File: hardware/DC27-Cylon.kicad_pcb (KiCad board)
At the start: 2 copper layers, 79 x 102 mm, 3 parts

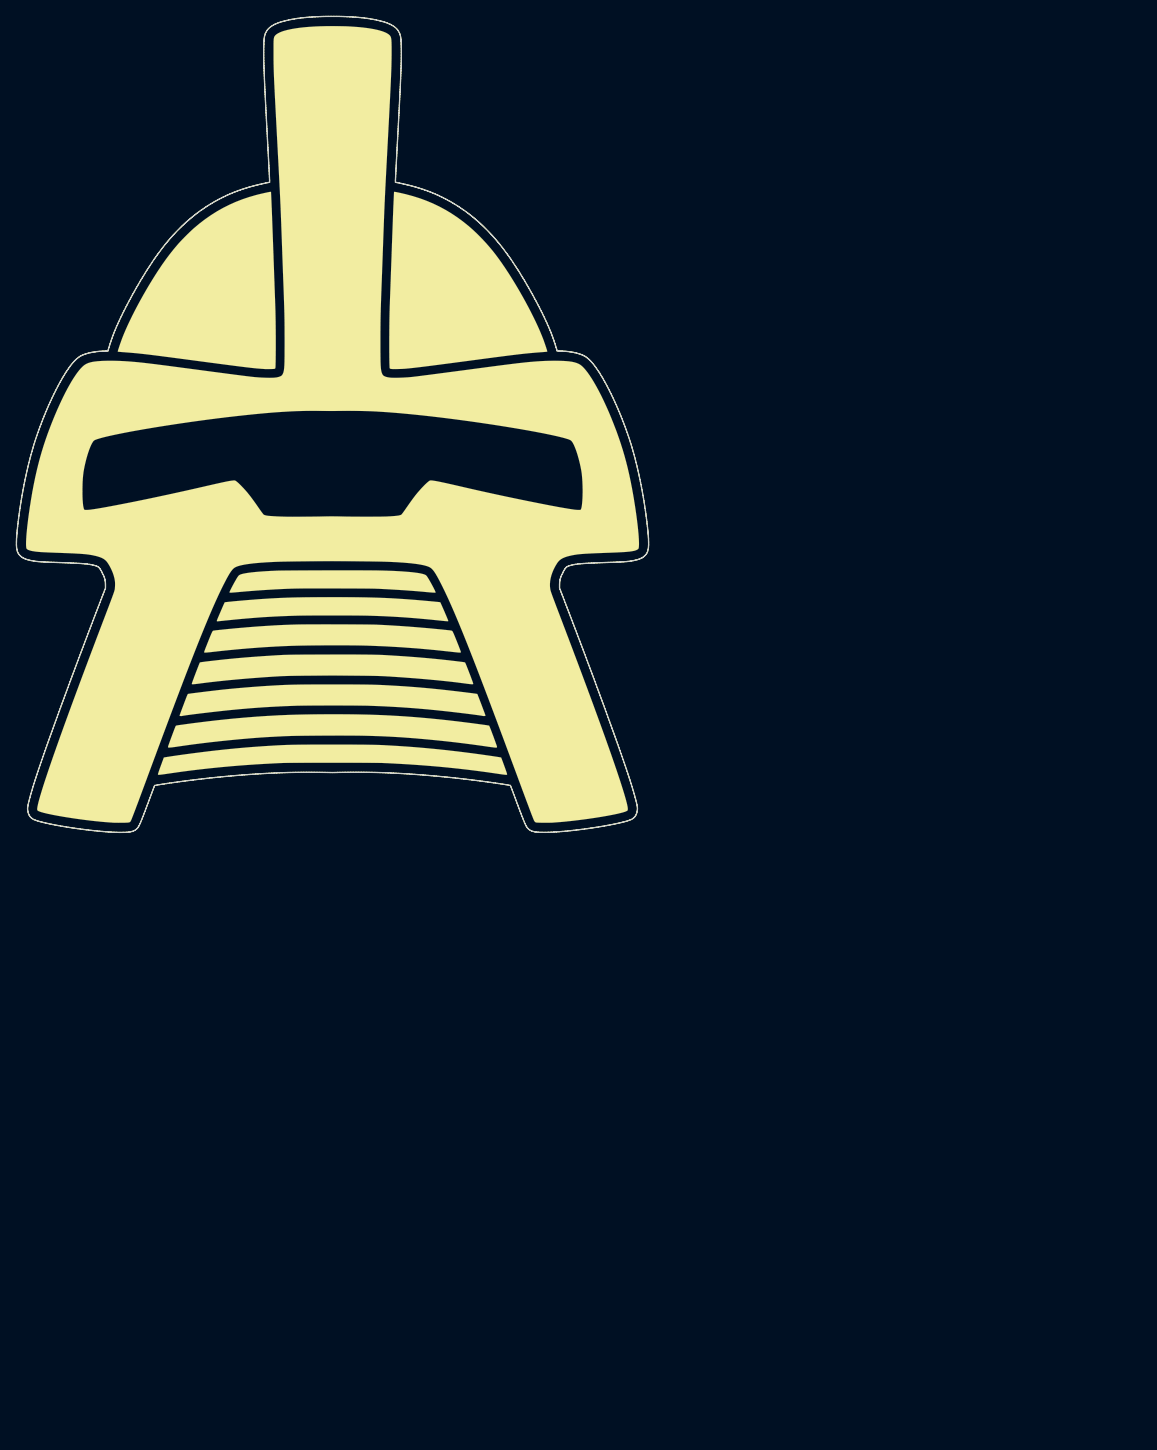
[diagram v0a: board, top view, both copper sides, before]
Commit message: Rough layout, still need all tracks
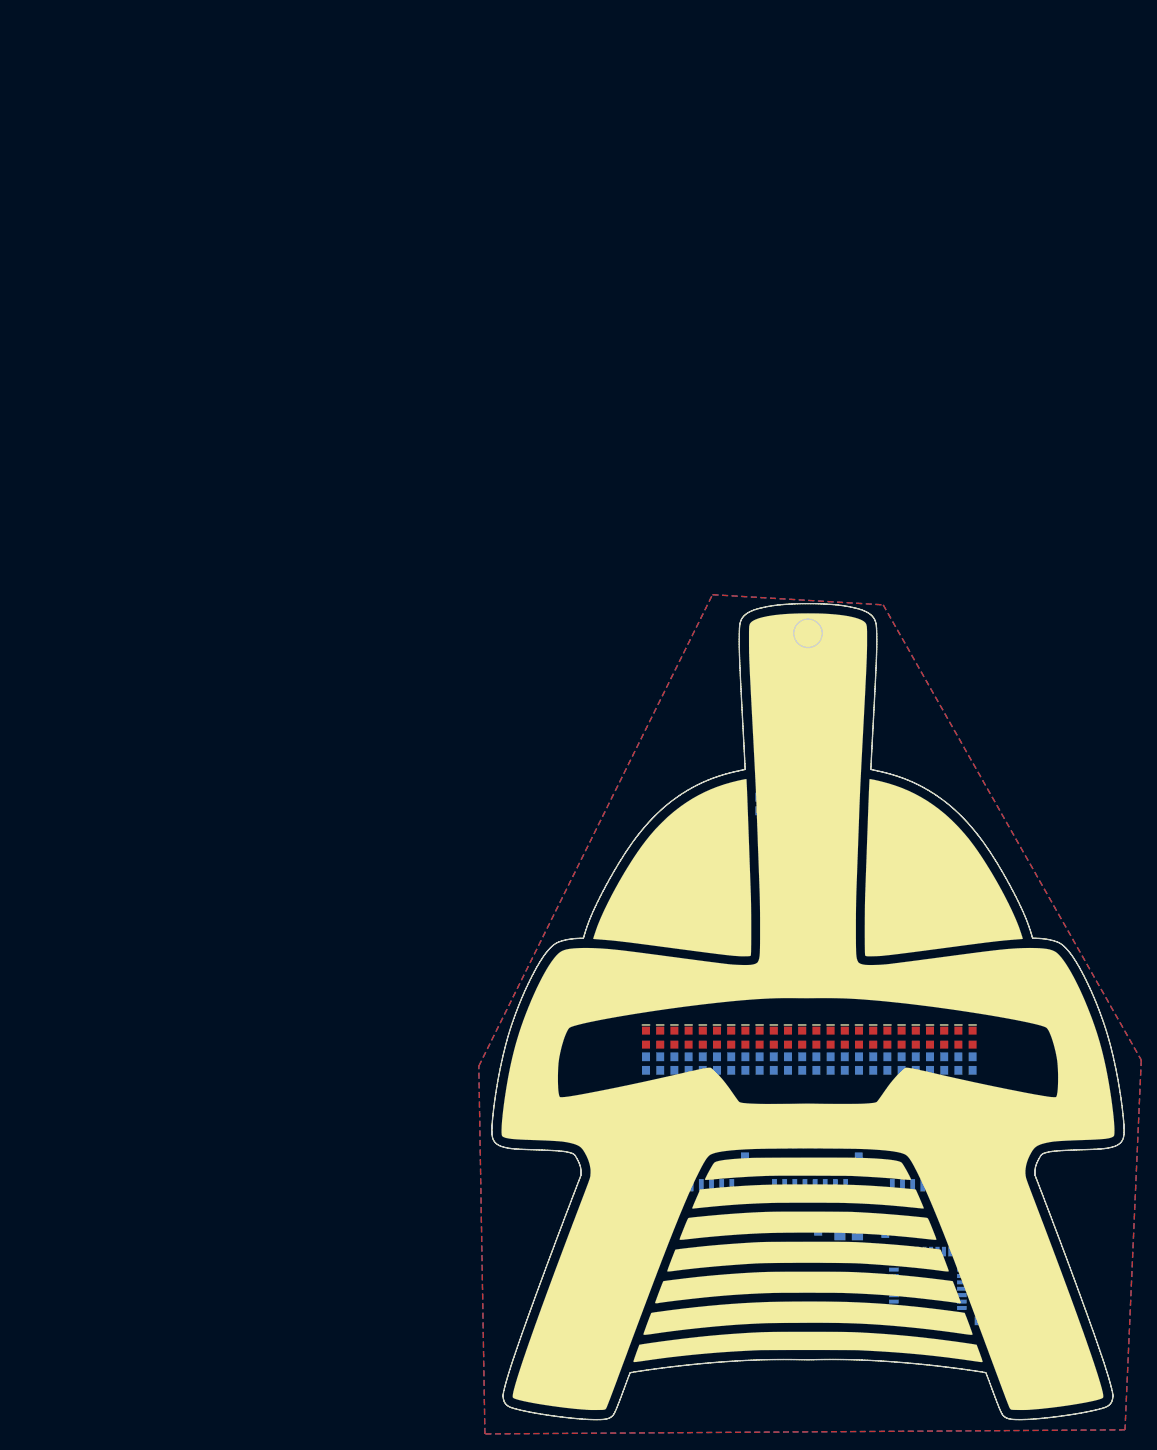
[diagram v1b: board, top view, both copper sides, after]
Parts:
- removed the G*** at (0.00, 0.00) (x3)
- added BT1: Battery, DC27-Cylon:BatteryHolder_Keystone_2464_3xAA, B.Cu at (44.2, 58.8)
- added C1: 22p, Sparkfun_Capacitors:0603, B.Cu at (60.7, 99.6)
- added C2: 10μ, Sparkfun_Capacitors:0603, B.Cu at (53.3, 47.0)
- added C3: 22p, Sparkfun_Capacitors:0603, B.Cu at (69.1, 99.8)
- added C4: 22p, Sparkfun_Capacitors:0603, B.Cu at (80.5, 91.9)
- added C5: 22p, Sparkfun_Capacitors:0603, B.Cu at (61.7, 43.2)
- added C6: 22p, Sparkfun_Capacitors:0603, B.Cu at (80.8, 110.7)
- added C7: 22p, Sparkfun_Capacitors:0603, B.Cu at (65.8, 91.9)
- added C8: 22p, Sparkfun_Capacitors:0603, B.Cu at (51.6, 91.9)
- added D1: LED0603, Sparkfun_LED:LED-0603, F.Cu at (80.0, 76.2)
- added D10: LED0603, Sparkfun_LED:LED-0603, F.Cu at (64.0, 76.2)
- added D11: LED0603, Sparkfun_LED:LED-0603, F.Cu at (62.3, 76.2)
- added D12: LED0603, Sparkfun_LED:LED-0603, F.Cu at (60.5, 76.2)
- added D13: LED0603, Sparkfun_LED:LED-0603, F.Cu at (58.7, 76.2)
- added D14: LED0603, Sparkfun_LED:LED-0603, F.Cu at (56.9, 76.2)
- added D15: LED0603, Sparkfun_LED:LED-0603, F.Cu at (55.2, 76.2)
- added D16: LED0603, Sparkfun_LED:LED-0603, F.Cu at (53.4, 76.2)
- added D17: LED0603, Sparkfun_LED:LED-0603, F.Cu at (51.6, 76.2)
- added D18: LED0603, Sparkfun_LED:LED-0603, F.Cu at (49.8, 76.2)
- added D19: LED0603, Sparkfun_LED:LED-0603, F.Cu at (48.1, 76.2)
- added D2: LED0603, Sparkfun_LED:LED-0603, F.Cu at (78.2, 76.2)
- added D20: LED0603, Sparkfun_LED:LED-0603, F.Cu at (46.3, 76.2)
- added D21: LED0603, Sparkfun_LED:LED-0603, F.Cu at (44.5, 76.2)
- added D22: LED0603, Sparkfun_LED:LED-0603, F.Cu at (42.7, 76.2)
- added D23: LED0603, Sparkfun_LED:LED-0603, F.Cu at (41.0, 76.2)
- added D24: LED0603, Sparkfun_LED:LED-0603, F.Cu at (39.2, 76.2)
- added D3: LED0603, Sparkfun_LED:LED-0603, F.Cu at (76.5, 76.2)
- added D4: LED0603, Sparkfun_LED:LED-0603, F.Cu at (74.7, 76.2)
- added D5: LED0603, Sparkfun_LED:LED-0603, F.Cu at (72.9, 76.2)
- added D6: LED0603, Sparkfun_LED:LED-0603, F.Cu at (71.1, 76.2)
- added D7: LED0603, Sparkfun_LED:LED-0603, F.Cu at (69.4, 76.2)
- added D8: LED0603, Sparkfun_LED:LED-0603, F.Cu at (67.6, 76.2)
- added D9: LED0603, Sparkfun_LED:LED-0603, F.Cu at (65.8, 76.2)
- added G***: LOGO, LOGO, F.Cu at (0.00, 0.00)
- added G*** (x2): LOGO, LOGO, F.Cu at (59.4, 73.4)
- added ISP1: ISP, DC27-Cylon:ISP_2X3, B.Cu at (31.5, 110.5)
- added J1: CONN_04LOCK, Sparkfun_Connectors:1X04_LOCK, B.Cu at (93.5, 72.9)
- added J2: CONN_05LOCK, Sparkfun_Connectors:1X05_LOCK, B.Cu at (23.1, 81.8)
- added R1: 66.3, Sparkfun_Resistors:0603, B.Cu at (80.0, 79.4)
- added R10: 66.3, Sparkfun_Resistors:0603, B.Cu at (64.0, 79.4)
- added R11: 66.3, Sparkfun_Resistors:0603, B.Cu at (62.3, 79.4)
- added R12: 66.3, Sparkfun_Resistors:0603, B.Cu at (60.5, 79.4)
- added R13: 66.3, Sparkfun_Resistors:0603, B.Cu at (58.7, 79.4)
- added R14: 66.3, Sparkfun_Resistors:0603, B.Cu at (56.9, 79.4)
- added R15: 66.3, Sparkfun_Resistors:0603, B.Cu at (55.2, 79.4)
- added R16: 66.3, Sparkfun_Resistors:0603, B.Cu at (53.4, 79.4)
- added R17: 66.3, Sparkfun_Resistors:0603, B.Cu at (51.6, 79.4)
- added R18: 66.3, Sparkfun_Resistors:0603, B.Cu at (49.8, 79.4)
- added R19: 66.3, Sparkfun_Resistors:0603, B.Cu at (48.1, 79.4)
- added R2: 66.3, Sparkfun_Resistors:0603, B.Cu at (78.2, 79.4)
- added R20: 66.3, Sparkfun_Resistors:0603, B.Cu at (46.3, 79.4)
- added R21: 66.3, Sparkfun_Resistors:0603, B.Cu at (44.5, 79.4)
- added R22: 66.3, Sparkfun_Resistors:0603, B.Cu at (42.7, 79.4)
- added R23: 66.3, Sparkfun_Resistors:0603, B.Cu at (41.0, 79.4)
- added R24: 66.3, Sparkfun_Resistors:0603, B.Cu at (39.2, 79.4)
- added R3: 66.3, Sparkfun_Resistors:0603, B.Cu at (76.5, 79.4)
- added R4: 66.3, Sparkfun_Resistors:0603, B.Cu at (74.7, 79.4)
- added R5: 66.3, Sparkfun_Resistors:0603, B.Cu at (72.9, 79.4)
- added R6: 66.3, Sparkfun_Resistors:0603, B.Cu at (71.1, 79.4)
- added R7: 66.3, Sparkfun_Resistors:0603, B.Cu at (69.4, 79.4)
- added R8: 66.3, Sparkfun_Resistors:0603, B.Cu at (67.6, 79.4)
- added R9: 66.3, Sparkfun_Resistors:0603, B.Cu at (65.8, 79.4)
- added U1: STM32F030K6Tx, Digikey:LQFP-32_7x7mm, B.Cu at (74.4, 107.2)
- added U2: AZ1117-3.3, Package_TO_SOT_SMD:SOT-223-3_TabPin2, B.Cu at (59.4, 48.3)
- added U3: 74HC595D_118, Digikey:SOIC-16_W3.90mm, B.Cu at (74.4, 91.9)
- added U4: 74HC595D_118, Digikey:SOIC-16_W3.90mm, B.Cu at (59.7, 91.9)
- added U5: 74HC595D_118, Digikey:SOIC-16_W3.90mm, B.Cu at (45.5, 91.9)
- added Y1: 16MHz, DC27-Cylon:Crystal_SMD_3225-4Pin_3.2x2.5mm, B.Cu at (64.5, 100.1)
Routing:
- added copper zone on B.Cu, net +3V3
- added copper zone on F.Cu, net GND
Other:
- outline, holes or cut-outs redrawn
